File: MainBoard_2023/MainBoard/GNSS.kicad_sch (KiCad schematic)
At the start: 18 parts

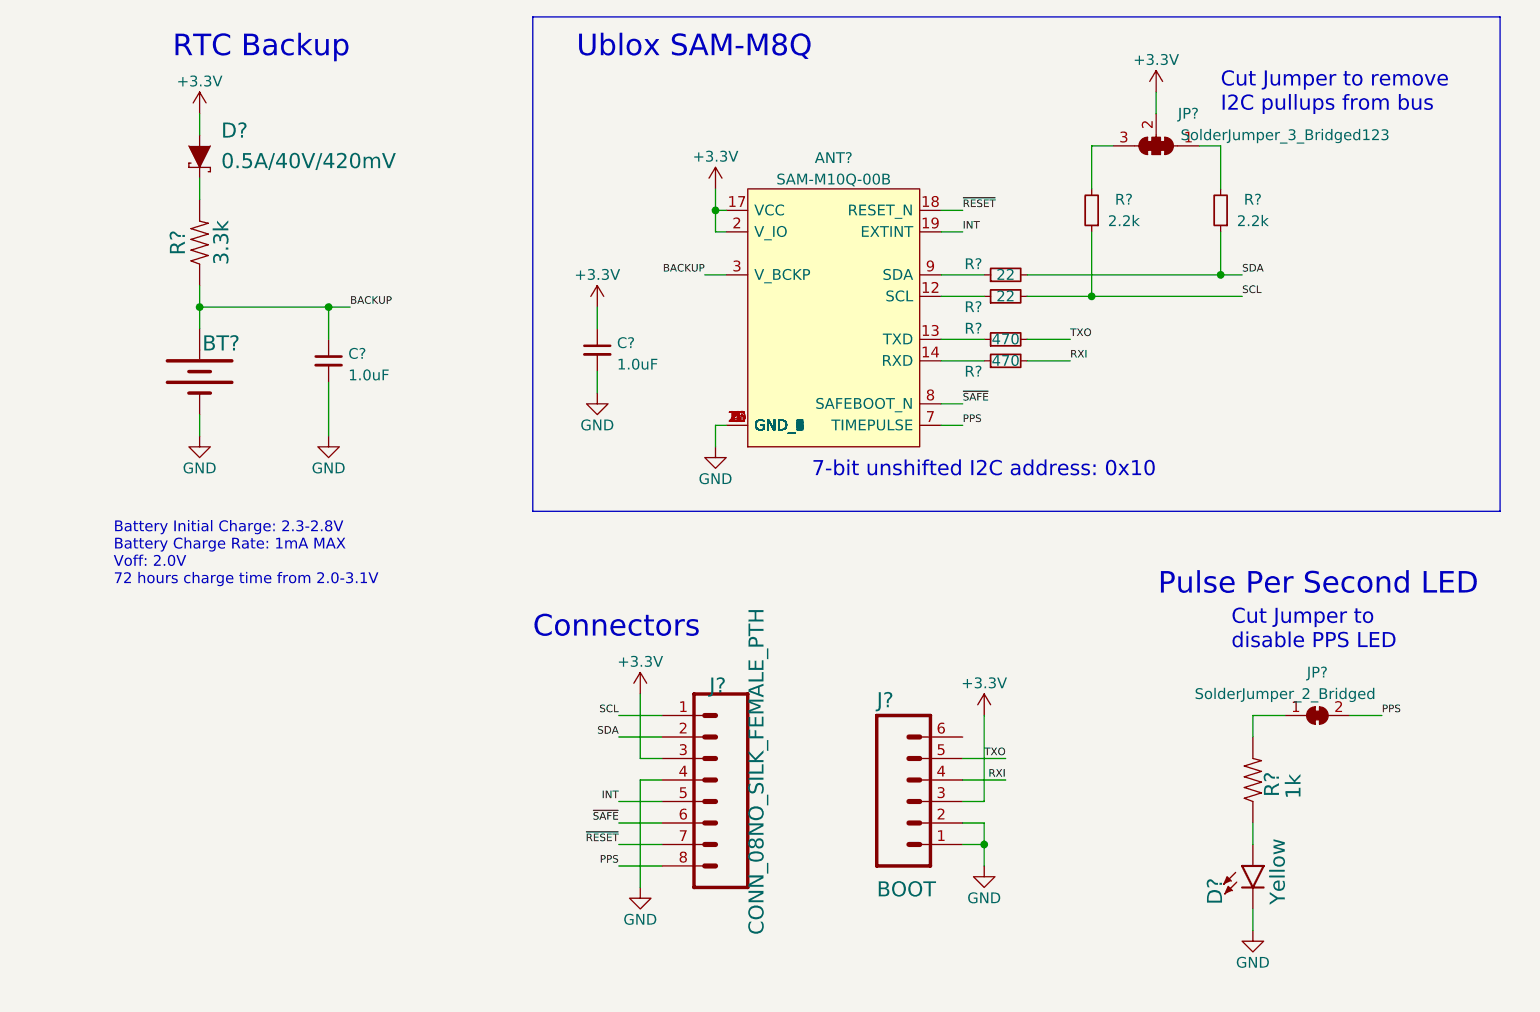
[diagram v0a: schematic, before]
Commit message: メイン基板設計一段落
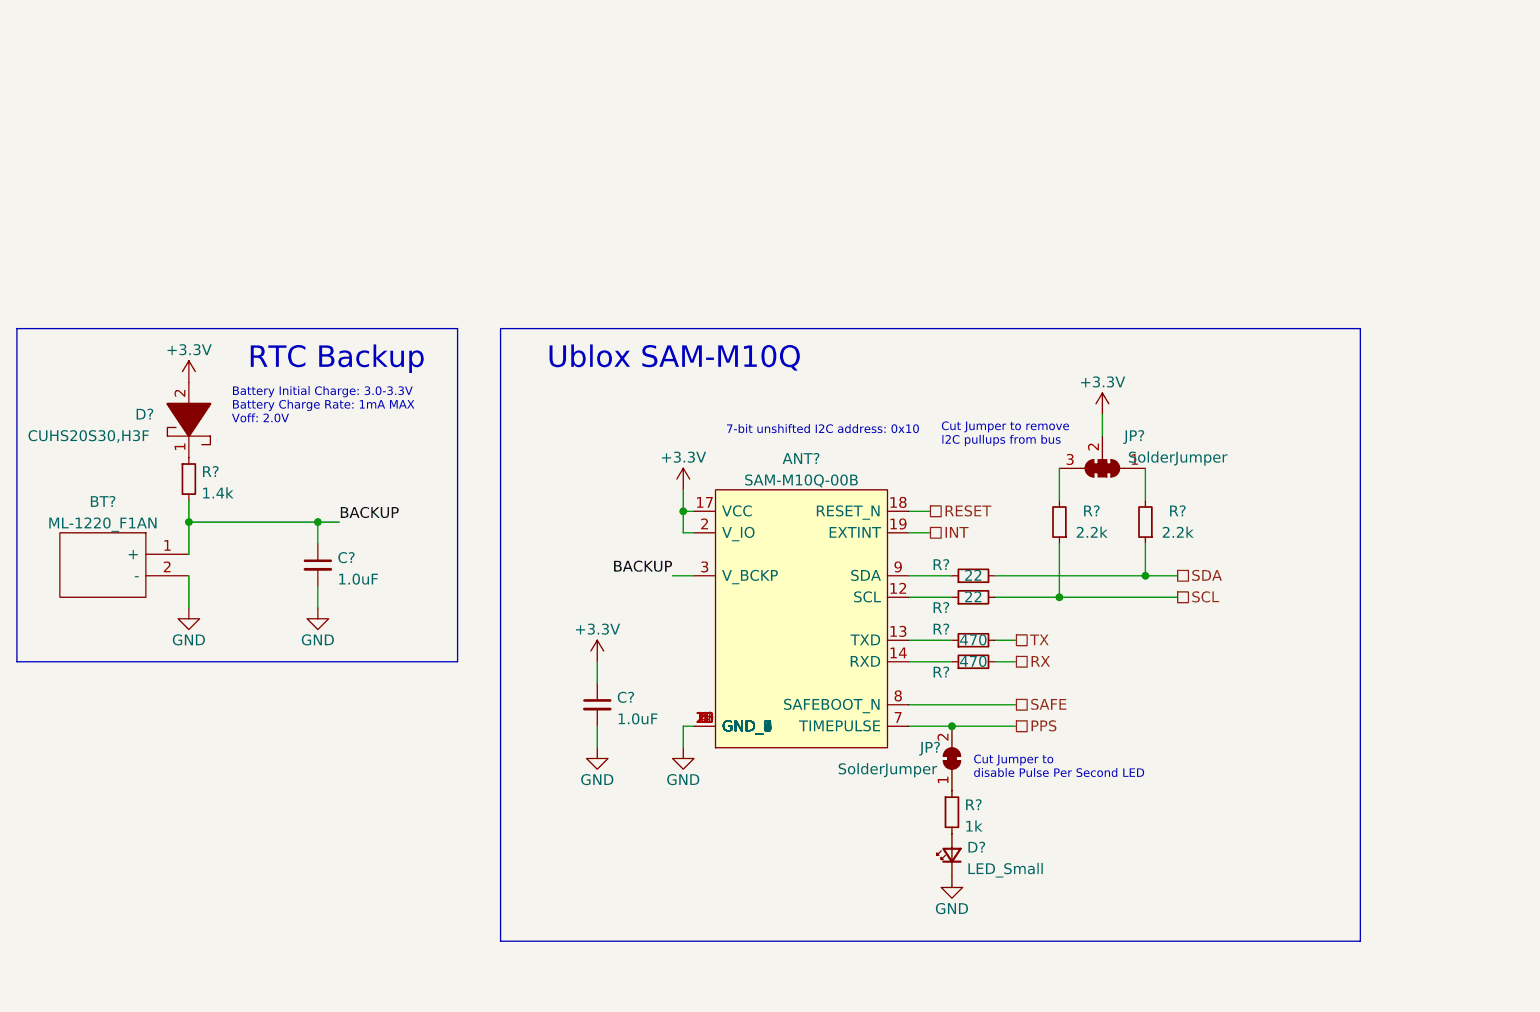
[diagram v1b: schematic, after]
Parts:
- removed BT?: 6.8MM_COIN_CELL, SparkFun_Ublox SAM-M8Q:ML414H_IV01E, symbol SparkFun_Ublox SAM-M8Q-eagle-import:ML414H_IV01E_BATTERY
- removed D?: Yellow, SparkFun_Ublox SAM-M8Q:LED-0603, symbol SparkFun_Ublox SAM-M8Q-eagle-import:LED-YELLOW0603
- removed D?: 0.5A/40V/420mV, SparkFun_Ublox SAM-M8Q:SOD-323, symbol SparkFun_Ublox SAM-M8Q-eagle-import:DIODE-SCHOTTKY-PMEG4005EJ
- removed J?: CONN_08NO_SILK_FEMALE_PTH, SparkFun_Ublox SAM-M8Q:1X08_NO_SILK, symbol SparkFun_Ublox SAM-M8Q-eagle-import:CONN_08NO_SILK_FEMALE_PTH
- removed J?: BOOT, SparkFun_Ublox SAM-M8Q:1X06_NO_SILK, symbol SparkFun_Ublox SAM-M8Q-eagle-import:CONN_06NO_SILK_NO_POP
- removed R?: 1k, SparkFun_Ublox SAM-M8Q:0603, symbol SparkFun_Ublox SAM-M8Q-eagle-import:1KOHM-0603-1/10W-1%
- removed R?: 3.3k, SparkFun_Ublox SAM-M8Q:0603, symbol SparkFun_Ublox SAM-M8Q-eagle-import:3.3KOHM-0603-1/10W-1%
- added BT?: ML-1220_F1AN, ML-1220F1AN, symbol ML-1220_F1AN:ML-1220_F1AN
- added D?: CUHS20S30,H3F, CUHS20S40H3F, symbol CUHS20S30:CUHS20S30,H3F
- added D?: LED_Small, symbol Device:LED_Small
- added R?: 1.4k, symbol Device:R_Small
- added R?: 1k, symbol Device:R_Small
- JP?: value SolderJumper_3_Bridged123 -> SolderJumper
- JP?: value SolderJumper_2_Bridged -> SolderJumper
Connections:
- net +3.3V: now also D?.2
- net BACKUP: now also BT?.1 (+), R?.2
- net GND: now also BT?.2 (-), D?.1 (K)
- net at JP?.1 (A): now also R?.1
- net RXI renamed RX
- net TXO renamed TX
- net ~{RESET} renamed RESET
- net ~{SAFE} renamed SAFE
- new net: D?.1, R?.1
- new net: D?.2 (A), R?.2
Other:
- note added: "Battery Initial Charge: 3.0-3.3V Battery Charge Rate: 1mA MAX Voff: 2.0V"
- note added: "Cut Jumper to disable Pulse Per Second LED"
- note added: "Ublox SAM-M10Q"
- note removed: "Battery Initial Charge: 2.3-2.8V Battery Charge Rate: 1mA MAX Voff: 2.0V 72 hours charge time from 2.0-3.1V"
- note removed: "Connectors"
- note removed: "Cut Jumper to disable PPS LED"
- note removed: "Pulse Per Second LED"
- note removed: "Ublox SAM-M8Q"
- moved on the sheet: ANT?, C?, JP?, R?
